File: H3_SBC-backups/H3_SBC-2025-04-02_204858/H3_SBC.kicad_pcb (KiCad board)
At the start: 6 copper layers, 50 x 40 mm, 14 parts, among them CN1 YXT-BB10-50P-02, CN2 YXT-BB10-50P-02, CN3 YXT-BB10-50P-02, Q1 WPM1481-6/TR, U1 H3, U10 XT28EG32GA4YJECGA, U2 AXP223_C2997893, U3 K4B4G1646E-BYMA 4GB, U4 K4B4G1646E-BYMA 4GB, U5 AP2127K-2.5, U9 RTL8211E-VB-CG, X1 X201232768KLD2SI, X2 SMD-5032_4P 24M 20pf, X3 5YAA25000121TF25E2

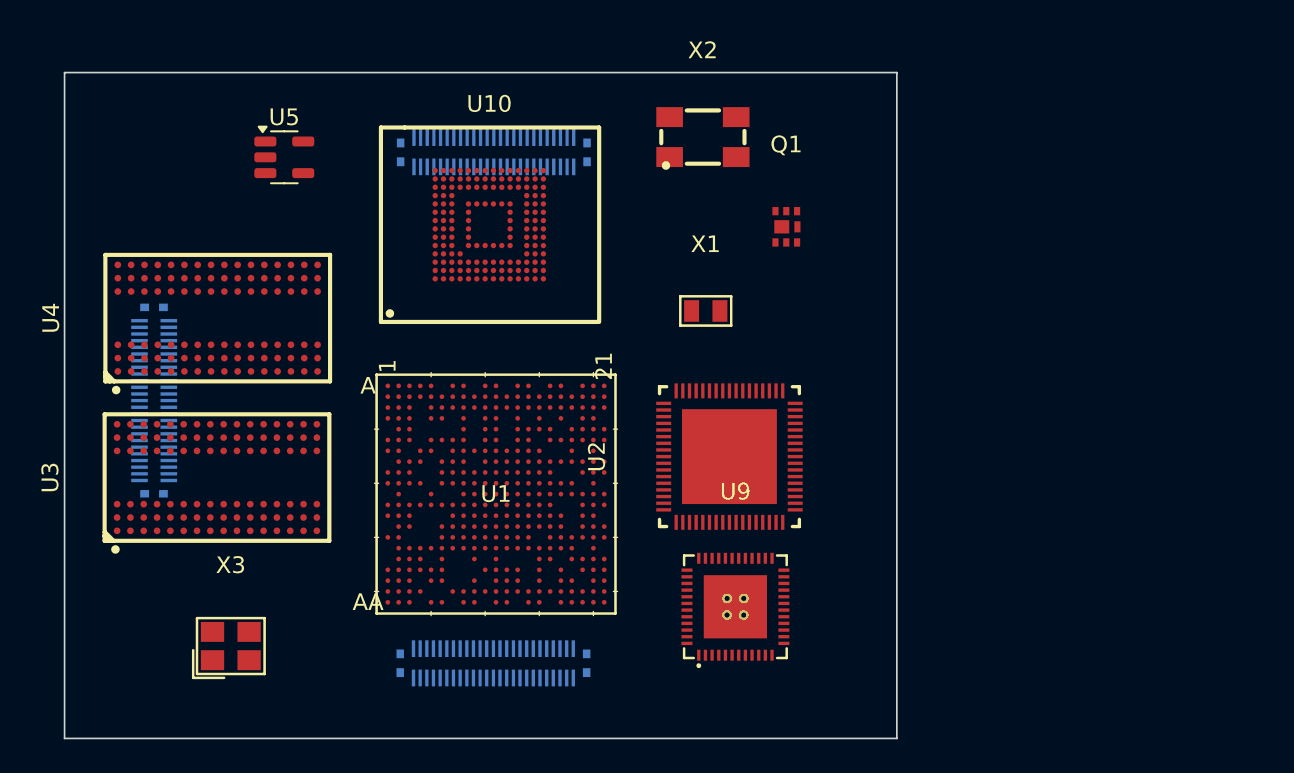
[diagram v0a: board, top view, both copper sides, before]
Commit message: small fixes
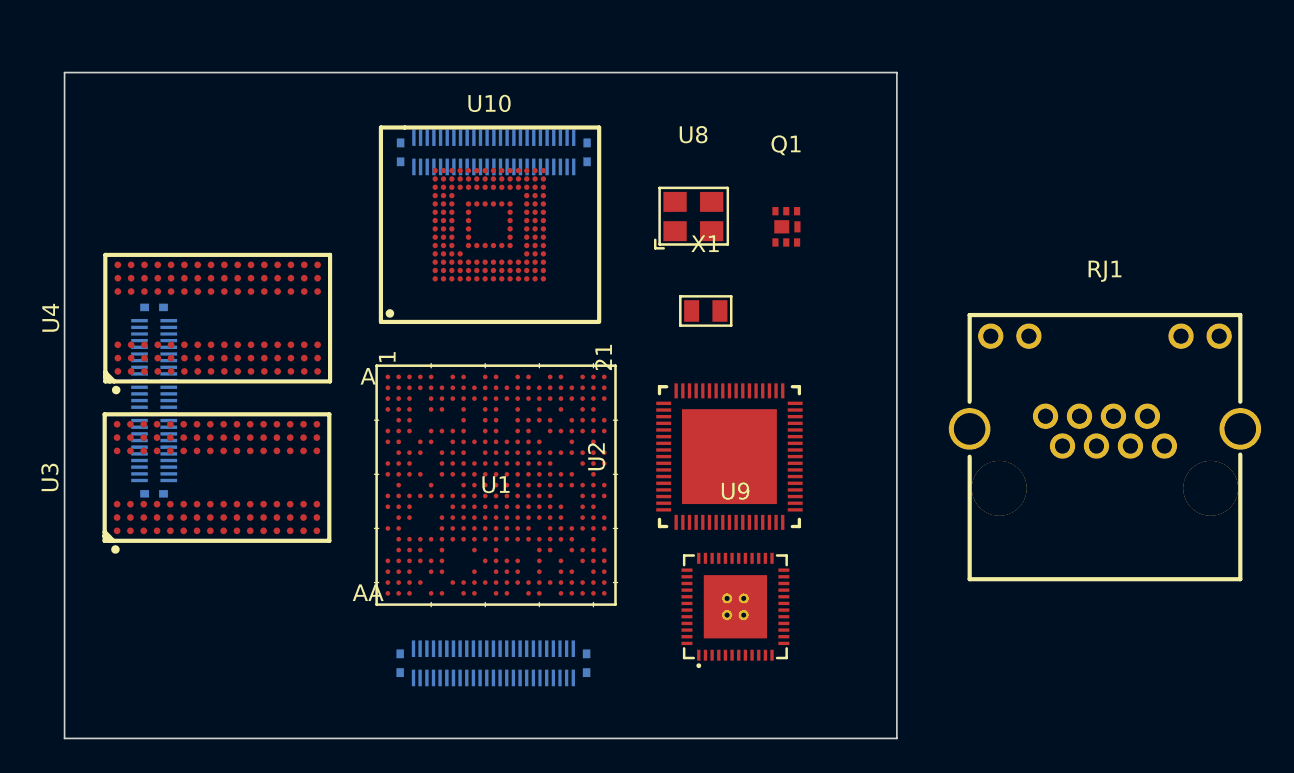
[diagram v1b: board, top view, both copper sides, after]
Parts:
- removed U5: AP2127K-2.5, Package_TO_SOT_SMD:SOT-23-5
- removed X2: SMD-5032_4P 24M 20pf, easyeda2kicad:CRYSTAL-SMD_4P-L5.0-W3.2-BL
- removed X3: 5YAA25000121TF25E2, easyeda2kicad:CRYSTAL-SMD_4P-L3.2-W2.5-BL
- added RJ1: R-RJ45R08P-C000, easyeda2kicad:RJ45-TH_R-RJ45R08P-C000, F.Cu at (212.5, 79.1)
- added U8: XOS32024000LT00351005, easyeda2kicad:OSC-SMD_4P-L3.2-W2.5-BL, F.Cu at (187.8, 68.6)
- moved U1 0.54 mm to (175.9, 84.8)
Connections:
- net VCC3V3_AUDIO renamed VCC_3V3_ANALOG
- CN1 pad 18: PG0 -> unconnected-(CN1-Pad18)
- CN1 pad 19: PG1 -> unconnected-(CN1-Pad19)
- CN1 pad 20: PG2 -> unconnected-(CN1-Pad20)
- CN1 pad 21: PG3 -> unconnected-(CN1-Pad21)
- CN1 pad 22: PG4 -> unconnected-(CN1-Pad22)
- CN1 pad 23: PG5 -> unconnected-(CN1-Pad23)
- CN1 pad 24: PG6 -> unconnected-(CN1-Pad24)
- CN1 pad 25: PG7 -> unconnected-(CN1-Pad25)
- CN2 pad 17: UBOOT -> unconnected-(CN2-Pad17)
- CN2 pad 18: GND -> unconnected-(CN2-Pad18)
- CN2 pad 19: PG8 -> unconnected-(CN2-Pad19)
- CN2 pad 20: PG9 -> unconnected-(CN2-Pad20)
- CN2 pad 21: GND -> unconnected-(CN2-Pad21)
- CN2 pad 22: DCDC4 -> unconnected-(CN2-Pad22)
- CN2 pad 23: DCDC4 -> unconnected-(CN2-Pad23)
- CN2 pad 24: DCDC4 -> unconnected-(CN2-Pad24)
- CN2 pad 25: DCDC4 -> unconnected-(CN2-Pad25)
- CN2 pad 37: GND -> unconnected-(CN2-Pad37)
- CN2 pad 38: PG11 -> unconnected-(CN2-Pad38)
- CN2 pad 39: PG10 -> unconnected-(CN2-Pad39)
- CN2 pad 40: GND -> unconnected-(CN2-Pad40)
- CN3 pad 22: GND -> unconnected-(CN3-Pad22)
- CN3 pad 23: TVOUT -> unconnected-(CN3-Pad23)
- CN3 pad 24: GND -> unconnected-(CN3-Pad24)
- CN3 pad 25: PG11 -> unconnected-(CN3-Pad25)
- U2 pad 28: CPUX_FB -> VCC1V2_CPU
- U2 pad 64: /Power/IPSOUT -> unconnected-(U2E-VIN4-Pad64)
- U2 pad 65: Net-(U2E-LX4) -> unconnected-(U2E-LX4-Pad65)
- U2 pad 66: GND -> unconnected-(U2E-PGND4-Pad66)
- U2 pad 67: DCDC4 -> unconnected-(U2E-DCDC4-Pad67)
- U2 pad 9: /Power/IPSOUT -> Net-(U2F-VIN5)
- U9 pad 20: Net-(U9-INTB) -> unconnected-(U9-INTB-Pad20)
- U9 pad 21: /Ethernet/DVDD25 -> unconnected-(U9-DVDD33-Pad21)
- U9 pad 29: /Ethernet/PHYRSTB -> unconnected-(U9-PHYRSTB-Pad29)
- U9 pad 33: Net-(U9-PMEB) -> unconnected-(U9-PMEB-Pad33)
- U9 pad 37: VCC3V3 -> unconnected-(U9-DVDD33-Pad37)
- U9 pad 38: VCC3V3 -> unconnected-(U9-ENSWREG-Pad38)
- U9 pad 41: VCC3V3 -> unconnected-(U9-AVDD33-Pad41)
- U9 pad 42: /Ethernet/CKXTAL_OUT -> unconnected-(U9-CKXTAL1-Pad42)
- U9 pad 43: /Ethernet/CKXTAL_IN -> unconnected-(U9-CKXTAL2-Pad43)
- U9 pad 46: Net-(U9-CLK125) -> unconnected-(U9-CLK125-Pad46)
- U9 pad 6: VCC3V3 -> unconnected-(U9-AVDD33-Pad6)
